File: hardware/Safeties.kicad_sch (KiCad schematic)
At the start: 9 parts, among them K4 FINDER-30.22, U14 74AUP1G32

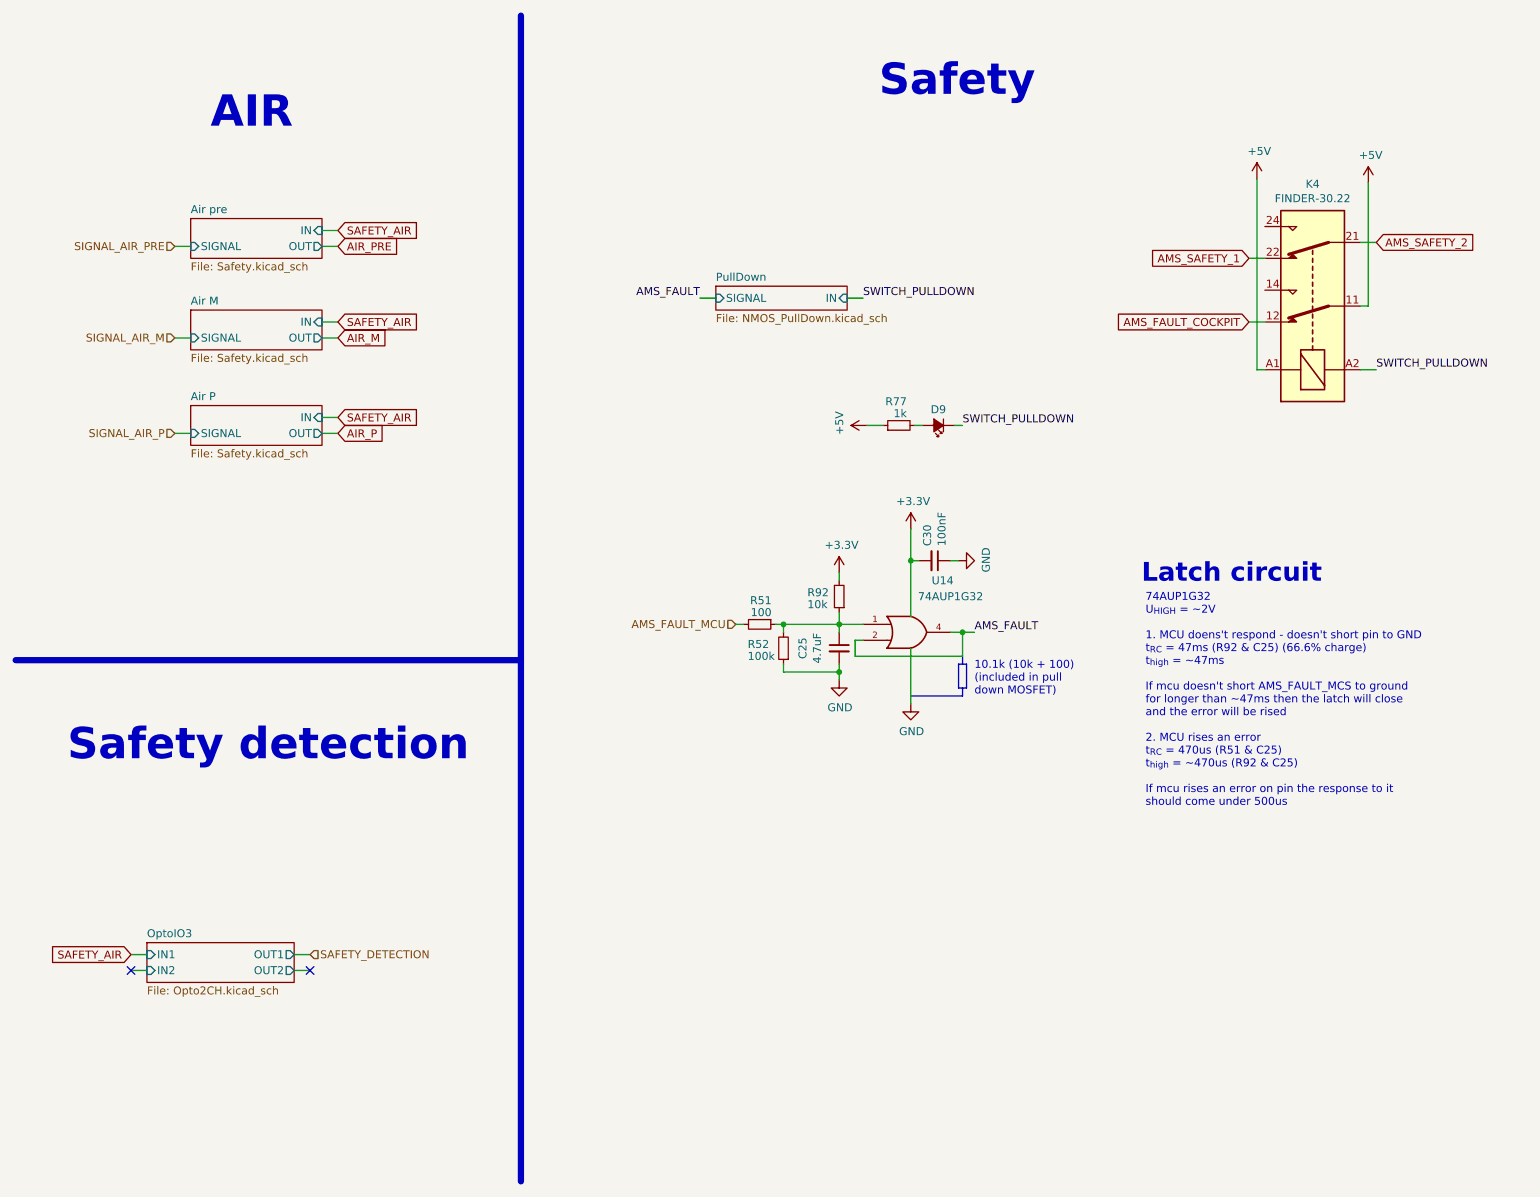
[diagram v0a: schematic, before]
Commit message: schematic override, just cuz
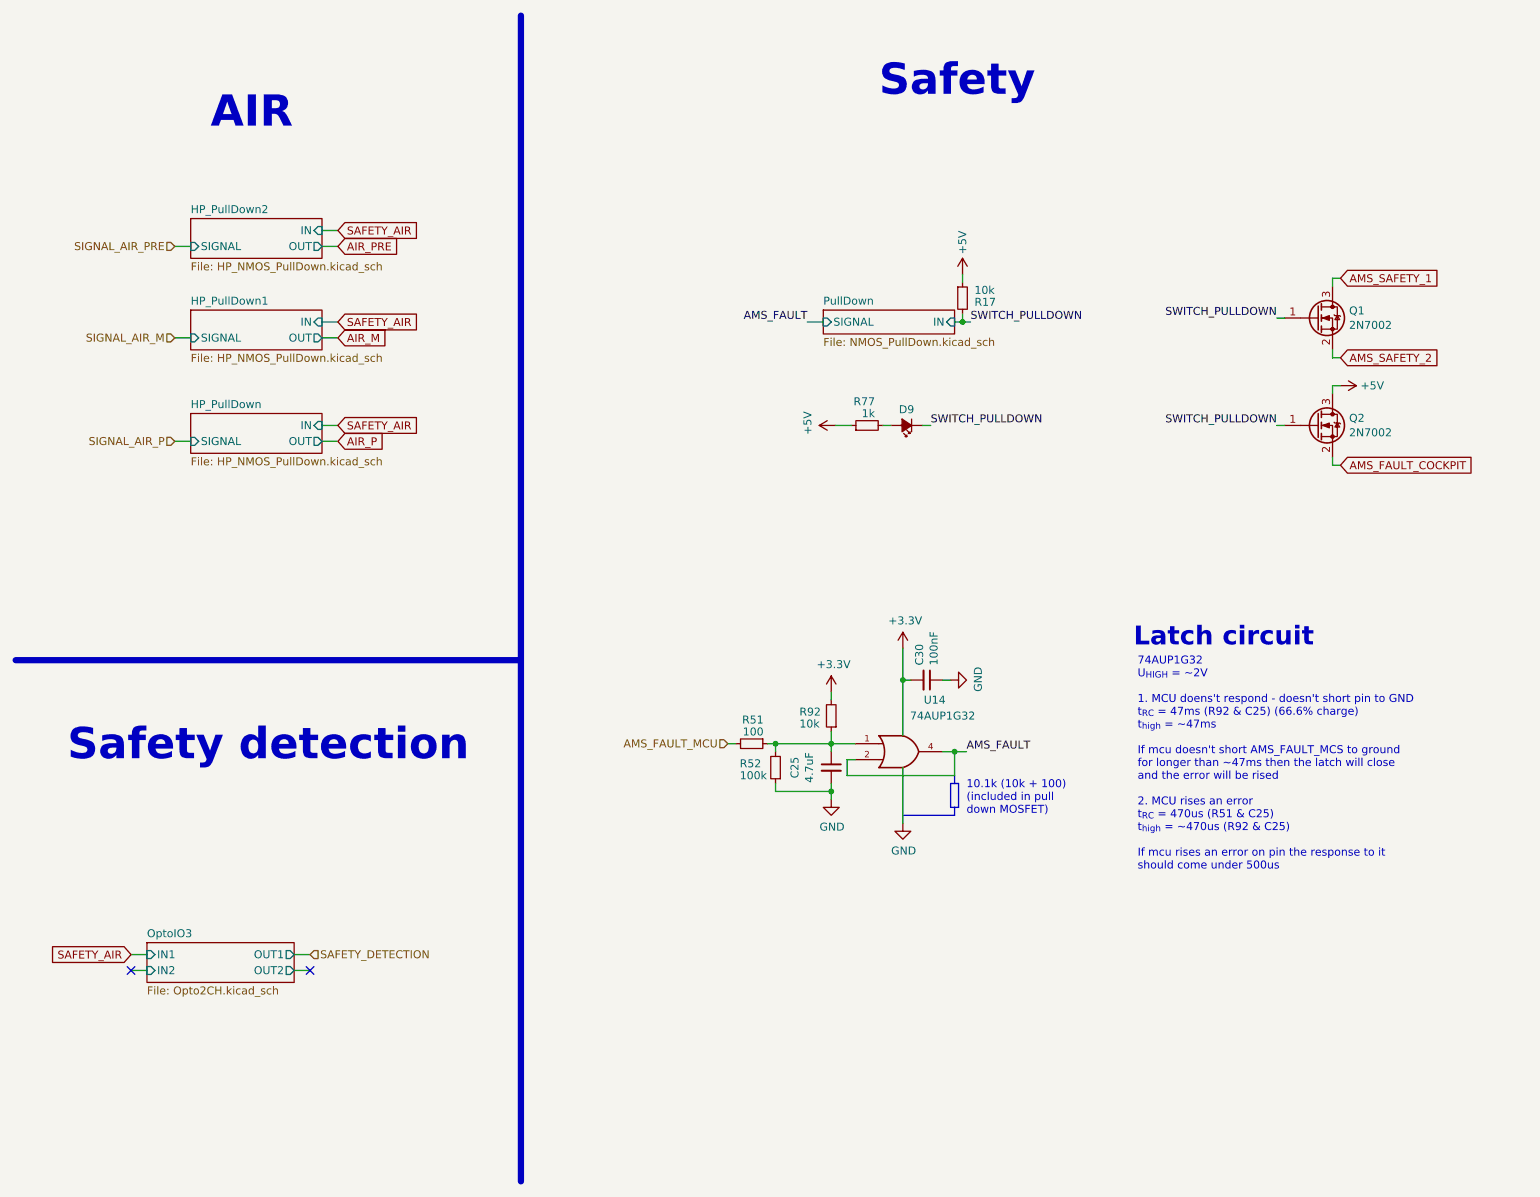
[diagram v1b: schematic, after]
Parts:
- removed K4: FINDER-30.22, Relay_THT:Relay_DPDT_Finder_30.22, symbol Relay:FINDER-30.22
- added Q1, Q2: 2N7002, Package_TO_SOT_SMD:SOT-23, symbol Transistor_FET:2N7002
- added R17: 10k, Resistor_SMD:R_0603_1608Metric, symbol Device:R_Small
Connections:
- net +5V: now also Q2.3 (D), R17.1
- net AMS_FAULT_COCKPIT: now also Q2.2 (S)
- net AMS_SAFETY_1: now also Q1.3 (D)
- net AMS_SAFETY_2: now also Q1.2 (S)
- net SWITCH_PULLDOWN: now also Q1.1 (G), Q2.1 (G), R17.2
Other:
- removed sheet Air M
- removed sheet Air P
- removed sheet Air pre
- added sheet HP_PullDown (HP_NMOS_PullDown.kicad_sch)
- added sheet HP_PullDown1 (HP_NMOS_PullDown.kicad_sch)
- added sheet HP_PullDown2 (HP_NMOS_PullDown.kicad_sch)
- moved on the sheet: C25, C30, D9, R51, R52, R77, R92, U14
